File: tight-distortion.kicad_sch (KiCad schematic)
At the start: 18 parts, among them J1 Barrel_Jack_Switch, J2 AudioJack_TRS, J3 AudioJack_TRS, J4 Conn_01x08, J5 power-module, SW2 SW_DPDT_x2

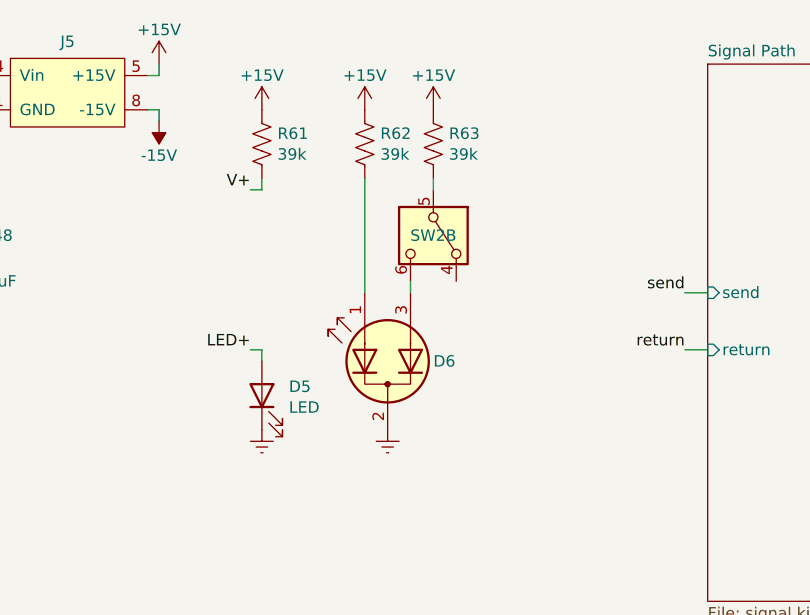
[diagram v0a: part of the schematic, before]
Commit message: small schematic change
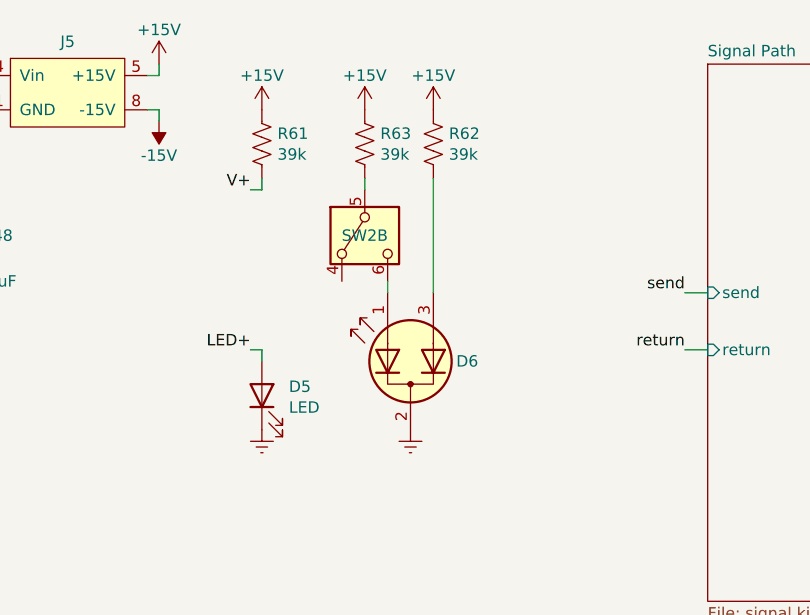
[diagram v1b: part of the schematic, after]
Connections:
- net at R62.2: now also D6.3 (A2); no longer D6.1 (A1)
- net at SW2.6 (C): now also D6.1 (A1); no longer D6.3 (A2)
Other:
- moved on the sheet: D6, R62, R63, SW2B
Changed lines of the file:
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@@
     (stroke (width 0) (type default))
   )
-  (wire (pts (xy 132.08 72.39) (xy 132.08 73.66))
+  (wire (pts (xy 129.54 72.39) (xy 129.54 73.66))
     (stroke (width 0) (type default))
   )
@@
     (stroke (width 0) (type default))
   )
-  (wire (pts (xy 134.62 62.23) (xy 134.62 60.96))
+  (wire (pts (xy 127 62.23) (xy 127 60.96))
     (stroke (width 0) (type default))
   )
@@
     (stroke (width 0) (type default))
   )
-  (wire (pts (xy 127 60.96) (xy 127 73.66))
+  (wire (pts (xy 134.62 60.96) (xy 134.62 73.66))
     (stroke (width 0) (type default))
   )
@@
     )
   )
-  (symbol (lib_id "power:Earth") (at 129.54 88.9 0) (unit 1)
-    (in_bom yes) (on_board yes) (dnp no)
-    (property "Reference" "#PWR068" (at 129.54 95.25 0)
-      (effects (font (size 1.27 1.27)) hide)
-    )
-    (property "Value" "Earth" (at 129.54 92.71 0)
-      (effects (font (size 1.27 1.27)) hide)
-    )
-    (property "Footprint" "" (at 129.54 88.9 0)
-      (effects (font (size 1.27 1.27)) hide)
-    )
-    (property "Datasheet" "~" (at 129.54 88.9 0)
+  (symbol (lib_id "power:Earth") (at 132.08 88.9 0) (mirror y) (unit 1)
+    (in_bom yes) (on_board yes) (dnp no)
+    (property "Reference" "#PWR068" (at 132.08 95.25 0)
+      (effects (font (size 1.27 1.27)) hide)
+    )
+    (property "Value" "Earth" (at 132.08 92.71 0)
+      (effects (font (size 1.27 1.27)) hide)
+    )
+    (property "Footprint" "" (at 132.08 88.9 0)
+      (effects (font (size 1.27 1.27)) hide)
+    )
+    (property "Datasheet" "~" (at 132.08 88.9 0)
       (effects (font (size 1.27 1.27)) hide)
     )
@@
     )
   )
-  (symbol (lib_id "bca-symbols:R") (at 127 57.15 270) (unit 1)
-    (in_bom yes) (on_board yes) (dnp no)
-    (property "Reference" "R62" (at 128.7272 55.9816 90)
-      (effects (font (size 1.27 1.27)) (justify left))
-    )
-    (property "Value" "39k" (at 128.7272 58.293 90)
-      (effects (font (size 1.27 1.27)) (justify left))
-    )
-    (property "Footprint" "bca-footprints:R_L3.6mm_D1.6mm_P5.00mm_Horizontal" (at 121.92 62.23 0)
-      (effects (font (size 1.27 1.27)) hide)
-    )
-    (property "Datasheet" "~" (at 127 57.15 90)
+  (symbol (lib_id "bca-symbols:R") (at 134.62 57.15 270) (unit 1)
+    (in_bom yes) (on_board yes) (dnp no)
+    (property "Reference" "R62" (at 136.3472 55.9816 90)
+      (effects (font (size 1.27 1.27)) (justify left))
+    )
+    (property "Value" "39k" (at 136.3472 58.293 90)
+      (effects (font (size 1.27 1.27)) (justify left))
+    )
+    (property "Footprint" "bca-footprints:R_L3.6mm_D1.6mm_P5.00mm_Horizontal" (at 129.54 62.23 0)
+      (effects (font (size 1.27 1.27)) hide)
+    )
+    (property "Datasheet" "~" (at 134.62 57.15 90)
       (effects (font (size 1.27 1.27)) hide)
     )
@@
     )
   )
-  (symbol (lib_id "bca-symbols:R") (at 134.62 57.15 270) (unit 1)
-    (in_bom yes) (on_board yes) (dnp no)
-    (property "Reference" "R63" (at 136.3472 55.9816 90)
-      (effects (font (size 1.27 1.27)) (justify left))
-    )
-    (property "Value" "39k" (at 136.3472 58.293 90)
-      (effects (font (size 1.27 1.27)) (justify left))
-    )
-    (property "Footprint" "bca-footprints:R_L3.6mm_D1.6mm_P5.00mm_Horizontal" (at 129.54 62.23 0)
-      (effects (font (size 1.27 1.27)) hide)
-    )
-    (property "Datasheet" "~" (at 134.62 57.15 90)
+  (symbol (lib_id "bca-symbols:R") (at 127 57.15 270) (unit 1)
+    (in_bom yes) (on_board yes) (dnp no)
+    (property "Reference" "R63" (at 128.7272 55.9816 90)
+      (effects (font (size 1.27 1.27)) (justify left))
+    )
+    (property "Value" "39k" (at 128.7272 58.293 90)
+      (effects (font (size 1.27 1.27)) (justify left))
+    )
+    (property "Footprint" "bca-footprints:R_L3.6mm_D1.6mm_P5.00mm_Horizontal" (at 121.92 62.23 0)
+      (effects (font (size 1.27 1.27)) hide)
+    )
+    (property "Datasheet" "~" (at 127 57.15 90)
       (effects (font (size 1.27 1.27)) hide)
     )
@@
     )
   )
-  (symbol (lib_id "Device:LED_Dual_AKA") (at 129.54 81.28 90) (unit 1)
-    (in_bom yes) (on_board yes) (dnp no)
-    (property "Reference" "D6" (at 134.62 81.28 90)
+  (symbol (lib_id "Device:LED_Dual_AKA") (at 132.08 81.28 90) (unit 1)
+    (in_bom yes) (on_board yes) (dnp no)
+    (property "Reference" "D6" (at 137.16 81.28 90)
       (effects (font (size 1.27 1.27)) (justify right))
     )
-    (property "Value" "LED_Dual_AAK" (at 135.89 82.4865 90)
+    (property "Value" "LED_Dual_AAK" (at 138.43 82.4865 90)
       (effects (font (size 1.27 1.27)) (justify right) hide)
     )
-    (property "Footprint" "bca-footprints:LED_D5.0mm-3" (at 129.54 81.28 0)
-      (effects (font (size 1.27 1.27)) hide)
-    )
-    (property "Datasheet" "~" (at 129.54 81.28 0)
+    (property "Footprint" "bca-footprints:LED_D5.0mm-3" (at 132.08 81.28 0)
+      (effects (font (size 1.27 1.27)) hide)
+    )
+    (property "Datasheet" "~" (at 132.08 81.28 0)
       (effects (font (size 1.27 1.27)) hide)
     )
@@
     )
   )
-  (symbol (lib_id "power:+15V") (at 127 53.34 0) (unit 1)
-    (in_bom yes) (on_board yes) (dnp no)
-    (property "Reference" "#PWR067" (at 127 57.15 0)
-      (effects (font (size 1.27 1.27)) hide)
-    )
-    (property "Value" "+15V" (at 127 49.53 0)
-      (effects (font (size 1.27 1.27)))
-    )
-    (property "Footprint" "" (at 127 53.34 0)
-      (effects (font (size 1.27 1.27)) hide)
-    )
-    (property "Datasheet" "" (at 127 53.34 0)
+  (symbol (lib_id "power:+15V") (at 134.62 53.34 0) (mirror y) (unit 1)
+    (in_bom yes) (on_board yes) (dnp no)
+    (property "Reference" "#PWR067" (at 134.62 57.15 0)
+      (effects (font (size 1.27 1.27)) hide)
+    )
+    (property "Value" "+15V" (at 134.62 49.53 0)
+      (effects (font (size 1.27 1.27)))
+    )
+    (property "Footprint" "" (at 134.62 53.34 0)
+      (effects (font (size 1.27 1.27)) hide)
+    )
+    (property "Datasheet" "" (at 134.62 53.34 0)
       (effects (font (size 1.27 1.27)) hide)
     )
@@
     )
   )
-  (symbol (lib_id "Switch:SW_DPDT_x2") (at 134.62 67.31 270) (unit 2)
-    (in_bom yes) (on_board yes) (dnp no)
-    (property "Reference" "SW2" (at 134.62 67.31 90)
-      (effects (font (size 1.27 1.27)))
-    )
-    (property "Value" "SW_DPDT_x2" (at 129.8448 68.453 90)
+  (symbol (lib_id "Switch:SW_DPDT_x2") (at 127 67.31 90) (mirror x) (unit 2)
+    (in_bom yes) (on_board yes) (dnp no)
+    (property "Reference" "SW2" (at 127 67.31 90)
+      (effects (font (size 1.27 1.27)))
+    )
+    (property "Value" "SW_DPDT_x2" (at 131.7752 68.453 90)
       (effects (font (size 1.27 1.27)) (justify right) hide)
     )
-    (property "Footprint" "bca-footprints:Pin_Header_Straight_1x06_Pitch2.54mm" (at 134.62 67.31 0)
-      (effects (font (size 1.27 1.27)) hide)
-    )
-    (property "Datasheet" "~" (at 134.62 67.31 0)
+    (property "Footprint" "bca-footprints:Pin_Header_Straight_1x06_Pitch2.54mm" (at 127 67.31 0)
+      (effects (font (size 1.27 1.27)) hide)
+    )
+    (property "Datasheet" "~" (at 127 67.31 0)
       (effects (font (size 1.27 1.27)) hide)
     )
@@
     )
   )
-  (symbol (lib_id "power:+15V") (at 134.62 53.34 0) (unit 1)
-    (in_bom yes) (on_board yes) (dnp no)
-    (property "Reference" "#PWR069" (at 134.62 57.15 0)
-      (effects (font (size 1.27 1.27)) hide)
-    )
-    (property "Value" "+15V" (at 134.62 49.53 0)
-      (effects (font (size 1.27 1.27)))
-    )
-    (property "Footprint" "" (at 134.62 53.34 0)
-      (effects (font (size 1.27 1.27)) hide)
-    )
-    (property "Datasheet" "" (at 134.62 53.34 0)
-      (effects (font (size 1.27 1.27)) hide)
-    )
+  (symbol (lib_id "power:+15V") (at 127 53.34 0) (mirror y) (unit 1)
+    (in_bom yes) (on_board yes) (dnp no)
+    (property "Reference" "#PWR069" (at 127 57.15 0)
+      (effects (font (size 1.27 1.27)) hide)
+    )
+    (property "Value" "+15V" (at 127 49.53 0)
+      (effects (font (size 1.27 1.27)))
+    )
+    (property "Footprint" "" (at 127 53.34 0)
+      (effects (font (size 1.27 1.27)) hide)
+    )
+    (property "Datasheet" "" (at 127 53.34 0)
+      (effects (font (size 1.27 1.27)) hide)
+    )
